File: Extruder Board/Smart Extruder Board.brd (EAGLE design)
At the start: 36 x 30 mm, 17 parts

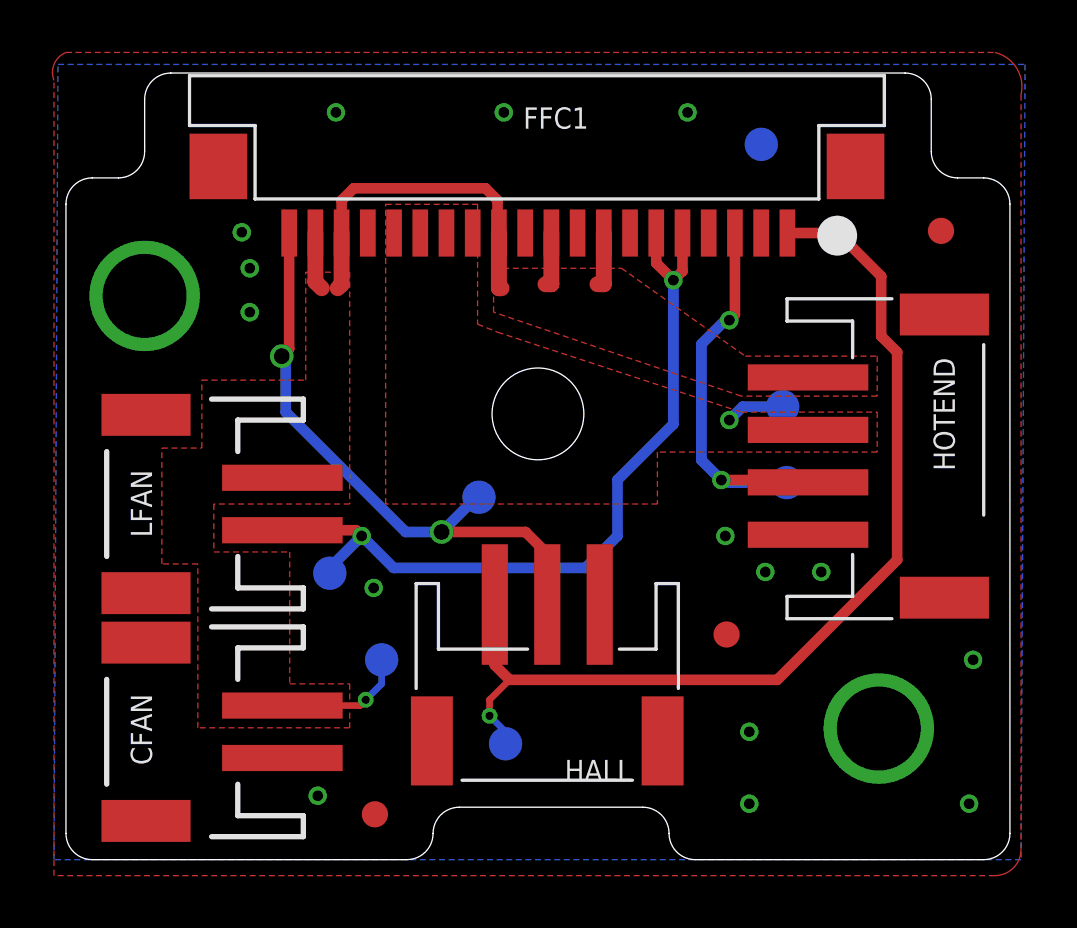
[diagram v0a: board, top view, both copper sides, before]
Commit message: BCN3D Electronics REV.E tested and manufactured
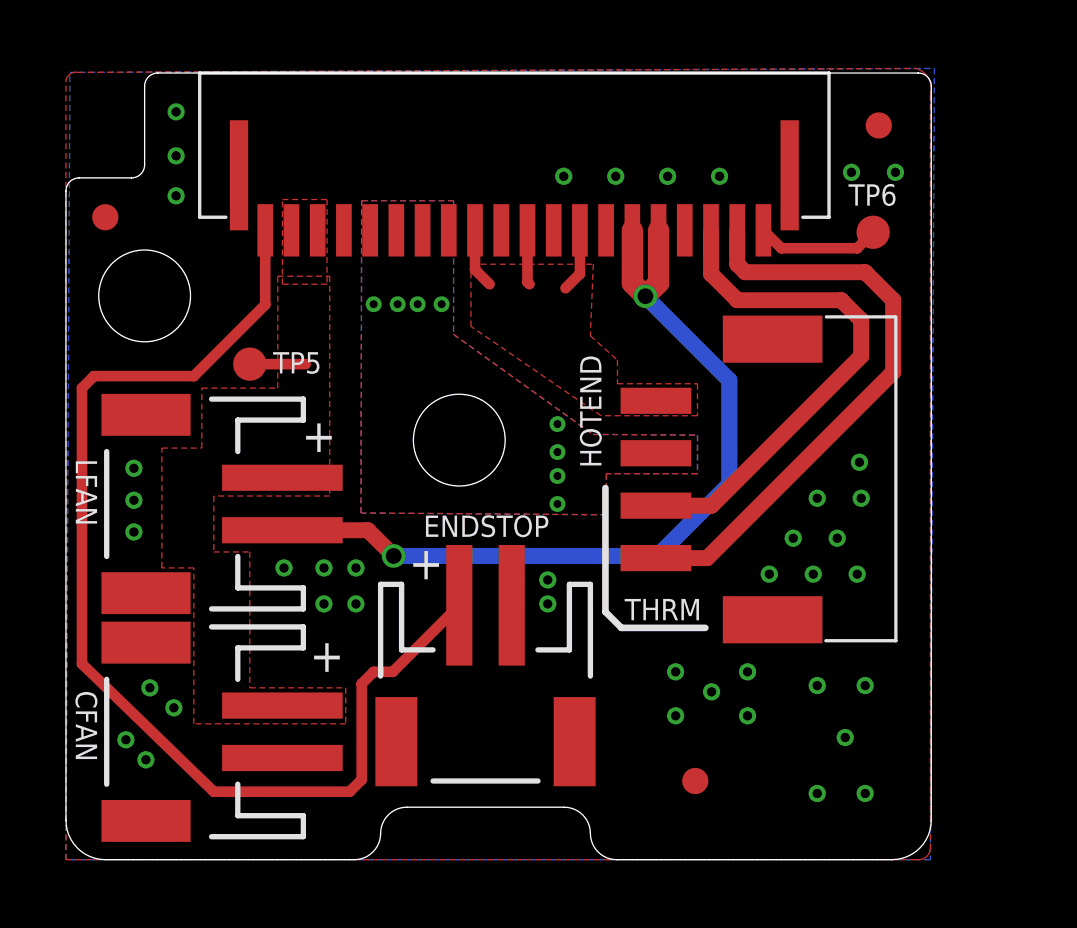
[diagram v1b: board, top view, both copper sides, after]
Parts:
- removed FFC1: FFC_20V_90G_1MM", MarcEagleParts:SAMTEC_ZF1-T-WT
- removed HALL: (no value), adafruit:JSTPH3
- removed HOTEND: (no value), MarcEagleParts:JSTPH3
- removed TP1, TP2, TP3, TP4, TP7: TPB1,27, testpad:B1,27
- added CN1: (no value), MarcEagleParts:JST_PA_04
- added ENDSTOP: (no value), SparkFun-Connectors:JST-2-SMD
- added U$6: (no value), MarcEagleParts:FCIM_LOGO
- added VERT_FFC1: FFC_20V_90G_1MM3, MarcEagleParts:FCI_20WAY_1MM_3ST
- moved U$3 25.0 mm to (1.50, 24.5)
- moved TP6 24.0 mm to (30.8, 23.9), flipped to the top, turned to 270 degrees
- moved TP5 12.3 mm to (7.01, 18.9), flipped to the top
- moved U$4 9.77 mm to (22.1, 4.47)
- moved U$2 5.71 mm to (24.0, 3.00)
- moved U$5 4.88 mm to (7.72, 6.78)
- moved U$1 4.67 mm to (31.0, 28.0)
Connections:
- removed net ATLVL: FFC1.20, HALL.2, TP4.TP
- new net GNDTHERM: CN1.4, VERT_FFC1.2
- new net Z-ENDSTOP: ENDSTOP.2, VERT_FFC1.20
- net +24V: now also CN1.1, VERT_FFC1.10, VERT_FFC1.12, VERT_FFC1.18, VERT_FFC1.19, VERT_FFC1.8; no longer FFC1.10, FFC1.12, FFC1.18, FFC1.19, FFC1.8, HOTEND.1
- net +5V: now also VERT_FFC1.1; no longer FFC1.1, HALL.3
- net GND: now also ENDSTOP.1, VERT_FFC1.11, VERT_FFC1.17, VERT_FFC1.4, VERT_FFC1.7, VERT_FFC1.9, VERT_FFC1.GND1, VERT_FFC1.GND2; no longer FFC1.11, FFC1.17, FFC1.2, FFC1.4, FFC1.7, FFC1.9, FFC1.GND1, FFC1.GND2, HALL.1, HOTEND.4, TP7.TP
- net HOTEND: now also CN1.2, VERT_FFC1.13, VERT_FFC1.14, VERT_FFC1.15, VERT_FFC1.16; no longer FFC1.13, FFC1.14, FFC1.15, FFC1.16, HOTEND.2, TP3.TP
- net HOTEND_THERM: now also CN1.3, VERT_FFC1.3; no longer FFC1.3, HOTEND.3, TP1.TP
- net LFAN: now also VERT_FFC1.5, VERT_FFC1.6; no longer FFC1.5, FFC1.6, TP2.TP
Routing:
- net Z-ENDSTOP: track 0.00 -> 43.1 mm
- net +5V: track 38.1 -> 4.72 mm, vias 1 -> 0
- net ATLVL: track 23.1 -> 0.00 mm, vias 2 -> 0
- net GNDTHERM: track 0.00 -> 22.5 mm
- net +24V: track 25.4 -> 8.94 mm, vias 1 -> 0
- net HOTEND_THERM: track 16.4 -> 19.7 mm, vias 2 -> 0
- net HOTEND: track 2.40 -> 0.00 mm, vias 1 -> 8
- net LFAN: track 30.5 -> 32.5 mm
- added copper zone on layer 16, net HOTEND
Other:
- board size 36 x 30 mm -> 33 x 30 mm
- board text added: "+"
- board text added: "BCN3D Electronics Extruder Board v1.0 Designed in Barcelona ___________________ May 2015 - REV_D"
- board text added: "HOTEND"
- board text added: "THRM"
- board text removed: "BCN3D Electronics çextruder Board v1.0 Designed in Barcelona ___________________ Extruder Board - Jan 2015 Marc Cobler - REV_B ___________________"
- board text removed: "Fundacio CIM"
